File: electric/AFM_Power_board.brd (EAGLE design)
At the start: 63.2 x 55.9 mm, 16 parts, among them IC1 LM4041CILP, IC2 LM7805_TO220V, IC3 7812T, J2 694103303002

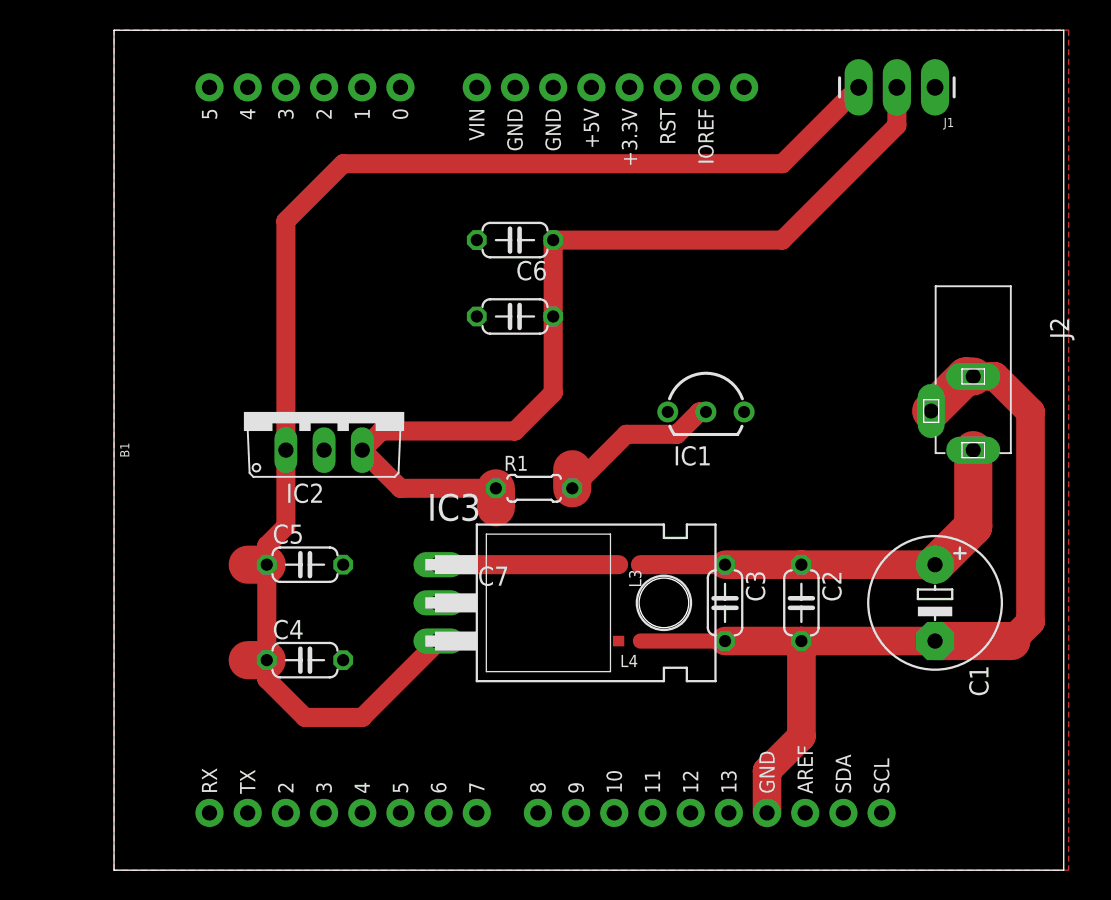
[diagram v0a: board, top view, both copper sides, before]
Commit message: allboards
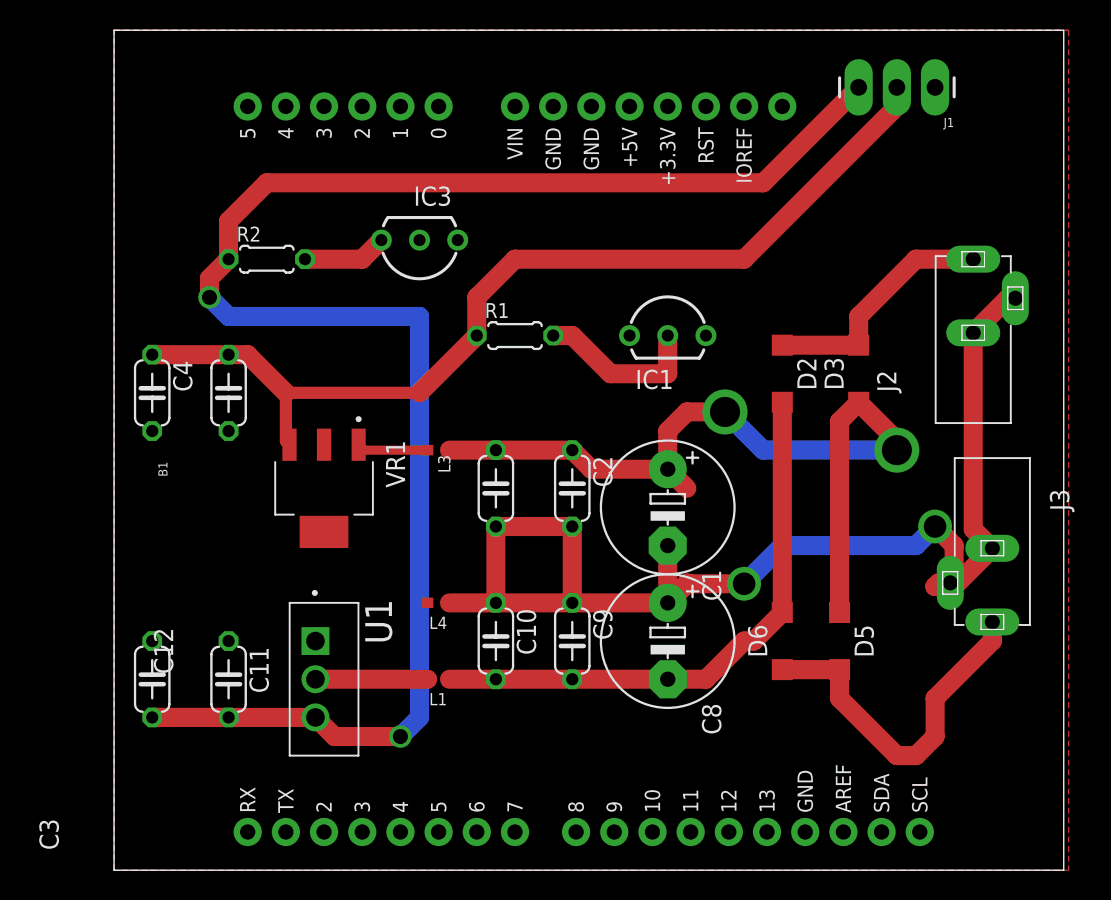
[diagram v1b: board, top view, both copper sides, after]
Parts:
- removed C6: 1uF, BeagleBone_Black_Wireless:C050-024X044
- removed C7: 10uF, BeagleBone_Black_Wireless:C050-024X044
- removed IC2: LM7805_TO220V, IC_Power-Management:TO220V
- added C10, C12: 1uF, BeagleBone_Black_Wireless:C050-024X044
- added C11, C9: 10uF, BeagleBone_Black_Wireless:C050-024X044
- added C8: 220uF, BeagleBone_Blue_R3:E5-8,5
- added D2, D3, D5, D6: 1n4004, diode:SOD123
- added J3: 694103303002, DC Power Jacks:694103303002
- added L1: 60Ohm@100 MHz, Wurth_EMC Components_WE-CBF:WE-CBF_0603_W2.2
- added R2: (no value), BeagleBone_Black_Wireless:0204/5
- added U1: LM7905CT/NOPB, LM7905CT_NOPB:TO254P1016X4575X1955-3
- added VR1: LM7805MP/NOPB, LM7805MP_NOPB:VREG_LM7805MP/NOPB
- IC3: value 7812T -> LM4041CILP; device adafruit:TO220H -> texas:LP_O-PBCY-W3
- moved IC3 26.7 mm to (20.3, 41.9), turned to 180 degrees
- moved C4 20.5 mm to (2.54, 31.8), turned to 270 degrees
- moved C1 18.9 mm to (36.8, 24.1)
- moved C2 17.0 mm to (30.5, 25.4)
- moved C3 17.0 mm to (25.4, 25.4)
- moved L3 14.8 mm to (21.6, 27.9)
- moved L4 13.0 mm to (21.6, 17.8)
- moved J2 12.7 mm to (57.1, 40.6), turned to 90 degrees
- moved C5 12.5 mm to (7.62, 31.8), turned to 270 degrees
- moved R1 10.2 mm to (26.7, 35.6)
- moved IC1 5.68 mm to (36.8, 35.6)
- moved B1 2.84 mm to (34.3, 26.7)
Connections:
- removed net N$3: IC3.1, L3.2
- removed net V12_OUT: C4.1, C5.1, IC2.1, IC3.3, J1.3
- new net GROUND: C1.-, C10.1, C2.2, C3.2, C8.+, C9.1, J2.2, J2.3, J3.2, J3.3, L4.1
- new net N$10: C10.2, C8.-, C9.2, D2.A, D6.A, L1.1
- new net N$11: C1.+, C2.1, C3.1, D3.C, D5.C, L3.1
- new net N$8: IC3.3, R2.2
- new net N$9: D5.A, D6.C, J3.1
- new net POWERP: D2.C, D3.A, J2.1
- new net VMINUS5_OUT: C11.2, C12.2, J1.3, R2.1, U1.3
- net AGND: now also B1.GND@0, B1.GND@1, B1.GND@2, C11.1, C12.1, U1.1, VR1.2, VR1.4; no longer C6.2, C7.2, IC2.2
- net N$1: now also L3.2, VR1.1; no longer C1.+, C2.1, C3.1, J2.1, L3.1
- net N$2: now also L1.2, U1.2; no longer B1.GND@2, C1.-, C2.2, C3.2, J2.2, J2.3, L4.1
- net V5_OUT: now also C4.1, C5.1, VR1.3; no longer C6.1, C7.1, IC2.3
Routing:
- net VMINUS5_OUT: track 0.00 -> 116.3 mm, vias 0 -> 2
- net V12_OUT: track 89.9 -> 0.00 mm
- net GROUND: track 0.00 -> 84.3 mm, vias 0 -> 2
- net N$11: track 0.00 -> 54.9 mm, vias 0 -> 2
- net N$2: track 61.4 -> 7.47 mm
- net N$10: track 0.00 -> 38.0 mm
- net N$1: track 28.3 -> 4.74 mm
- net N$9: track 0.00 -> 23.4 mm
- net POWERP: track 0.00 -> 16.2 mm
- net N$3: track 12.0 -> 0.00 mm
- net N$8: track 0.00 -> 5.61 mm
- net N$4: track 12.3 -> 11.2 mm
- net V5_OUT: track 64.2 -> 64.8 mm
